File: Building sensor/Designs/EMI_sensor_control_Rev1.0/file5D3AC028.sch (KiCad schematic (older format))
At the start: 5 parts, among them U10 ICE40LP8K-CM81

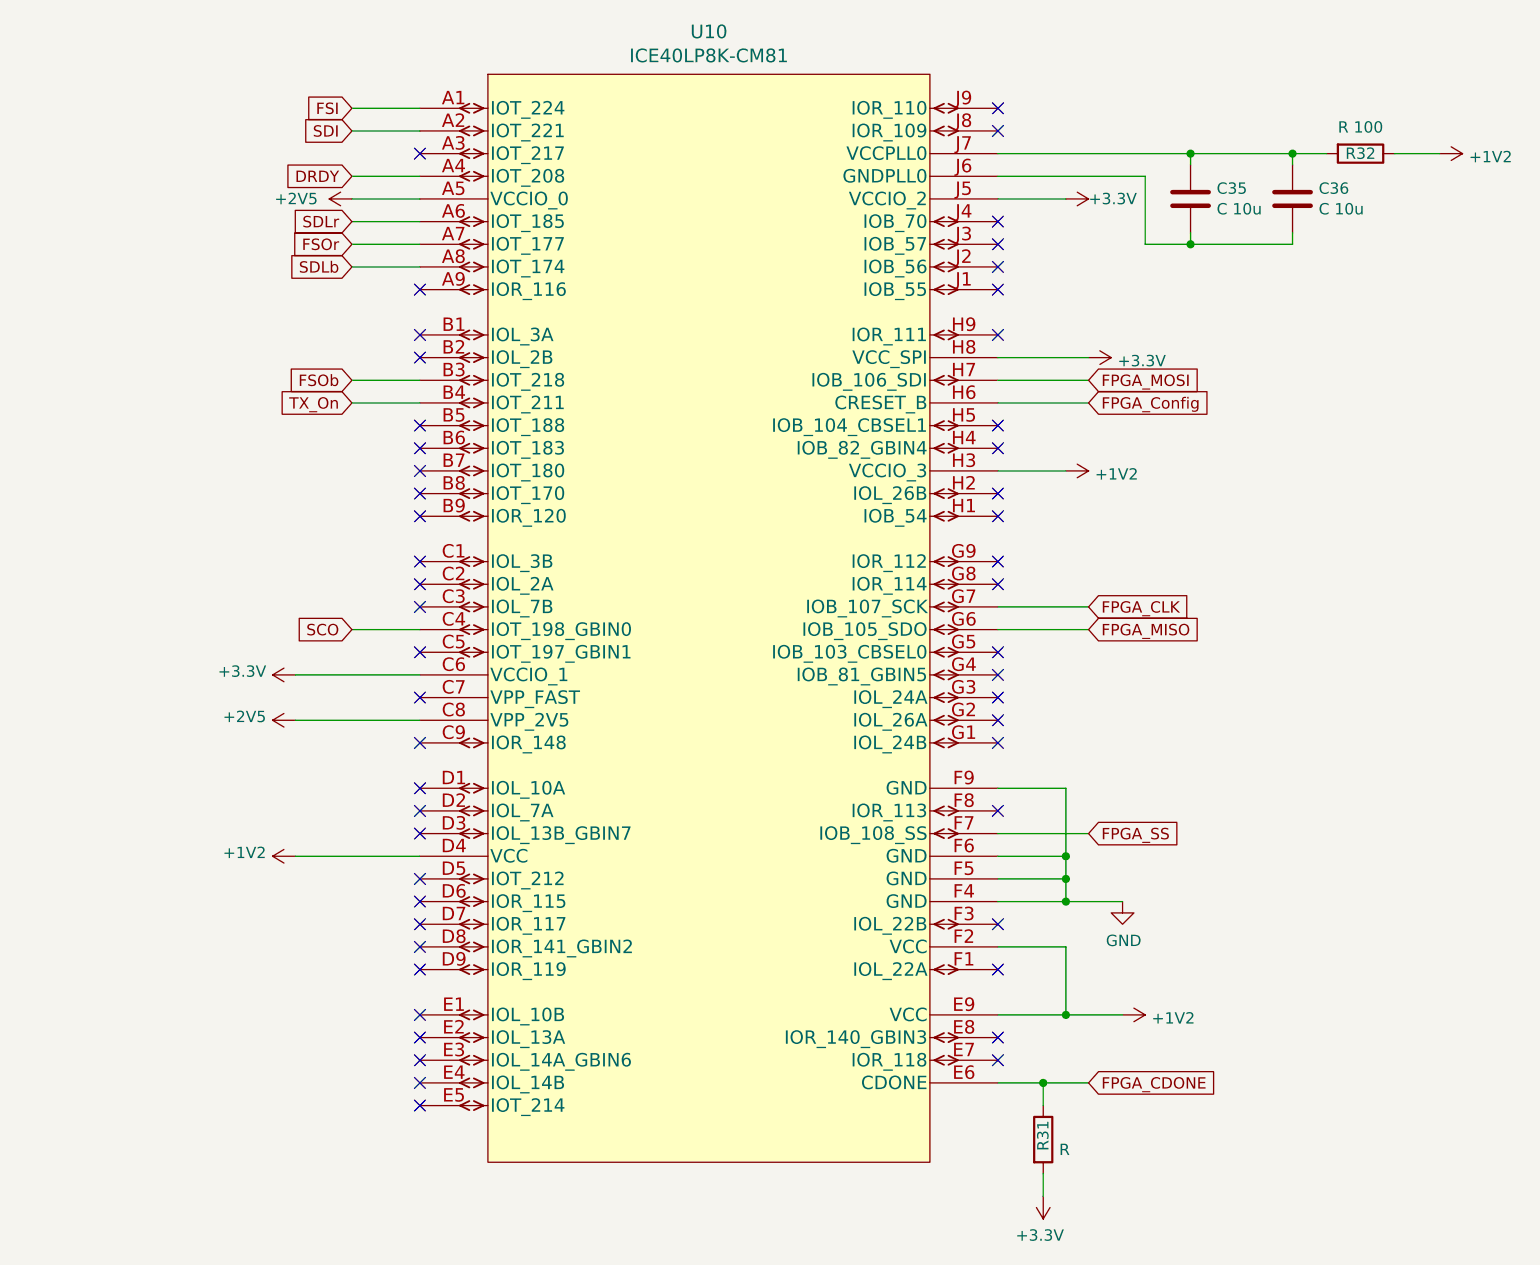
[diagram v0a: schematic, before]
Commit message: Weekly Commit
Weekly Commit 08/09/2019
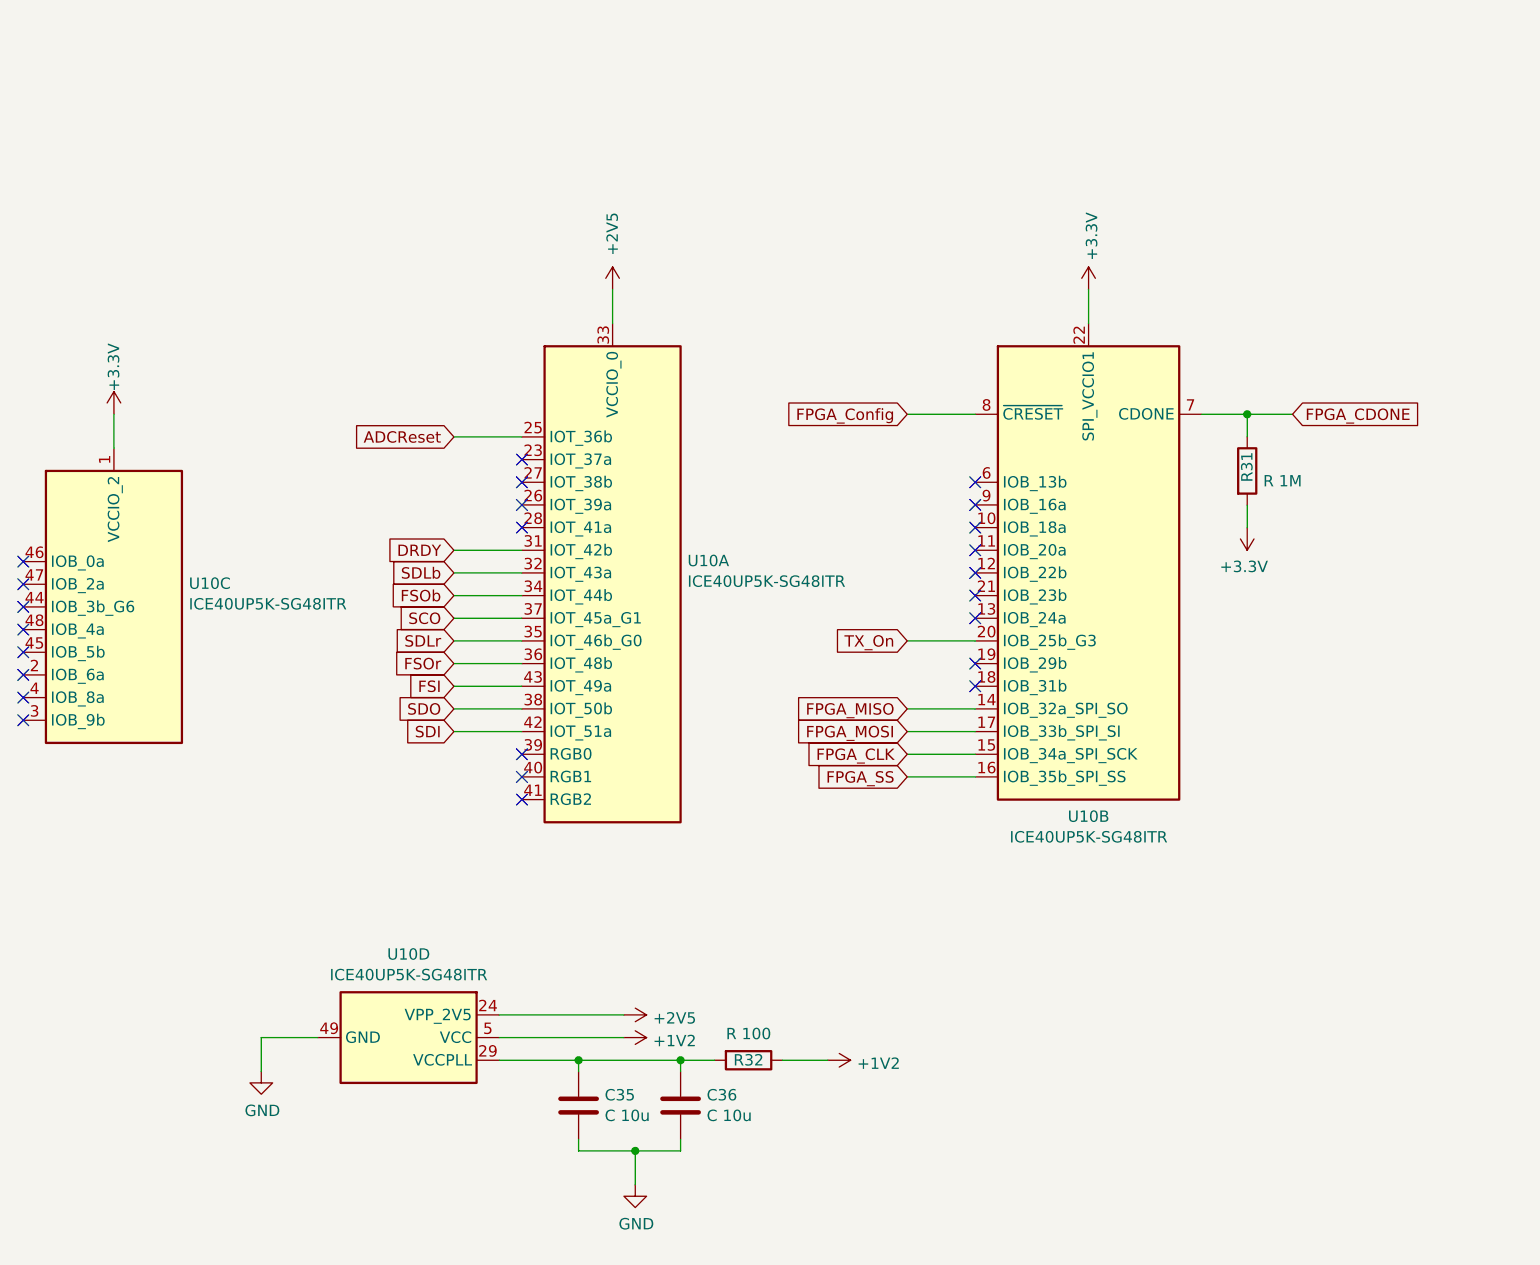
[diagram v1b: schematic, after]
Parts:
- removed U10: ICE40LP8K-CM81, ICE40UP5K-SG48ITR50:QFN50P700X700X100-49N, symbol 2019-07-24_19-23-14:ICE40LP8K-CM81
- added U10: ICE40UP5K-SG48ITR, Package_DFN_QFN:QFN-48-1EP_7x7mm_P0.5mm_EP5.6x5.6mm, symbol FPGA_Lattice:ICE40UP5K-SG48ITR
- R31: value R -> R 1M; footprint (none) -> Resistor_SMD:R_1206_3216Metric_Pad1.42x1.75mm_HandSolder
- R32: footprint (none) -> Resistor_SMD:R_1206_3216Metric_Pad1.42x1.75mm_HandSolder
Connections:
- net +1V2: now also U10.30 (VCC), U10.5 (VCC)
- net +2V5: now also U10.24 (VPP_2V5), U10.33 (VCCIO_0)
- net +3V3: now also U10.1 (VCCIO_2), U10.22 (SPI_VCCIO1)
- net DRDY: now also U10.31 (IOT_42b)
- net FPGA_CDONE: now also U10.7 (CDONE)
- net FPGA_CLK: now also U10.15 (IOB_34a_SPI_SCK)
- net FPGA_Config: now also U10.8 (~CRESET)
- net FPGA_MISO: now also U10.14 (IOB_32a_SPI_SO)
- net FPGA_MOSI: now also U10.17 (IOB_33b_SPI_SI)
- net FPGA_SS: now also U10.16 (IOB_35b_SPI_SS)
- net FSI: now also U10.43 (IOT_49a)
- net FSOb: now also U10.34 (IOT_44b)
- net FSOr: now also U10.36 (IOT_48b)
- net GND: now also C35.2, C36.2, U10.49 (GND)
- net SCO: now also U10.37 (IOT_45a_G1)
- net SDI: now also U10.42 (IOT_51a)
- net SDLb: now also U10.32 (IOT_43a)
- net SDLr: now also U10.35 (IOT_46b_G0)
- net TX_On: now also U10.20 (IOB_25b_G3)
- net at C35.1, C36.1, R32.2: now also U10.29 (VCCPLL)
- new net ADCReset: U10.25 (IOT_36b)
- new net SDO: U10.38 (IOT_50b)
- no-connect marks 51 -> 24
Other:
- moved on the sheet: C35, C36, R31, R32
